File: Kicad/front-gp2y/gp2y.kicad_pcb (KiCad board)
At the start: 2 copper layers, 48 x 35 mm, 16 parts, among them IC1 MCP1755-50, K1 GP2Y, K2 MCU

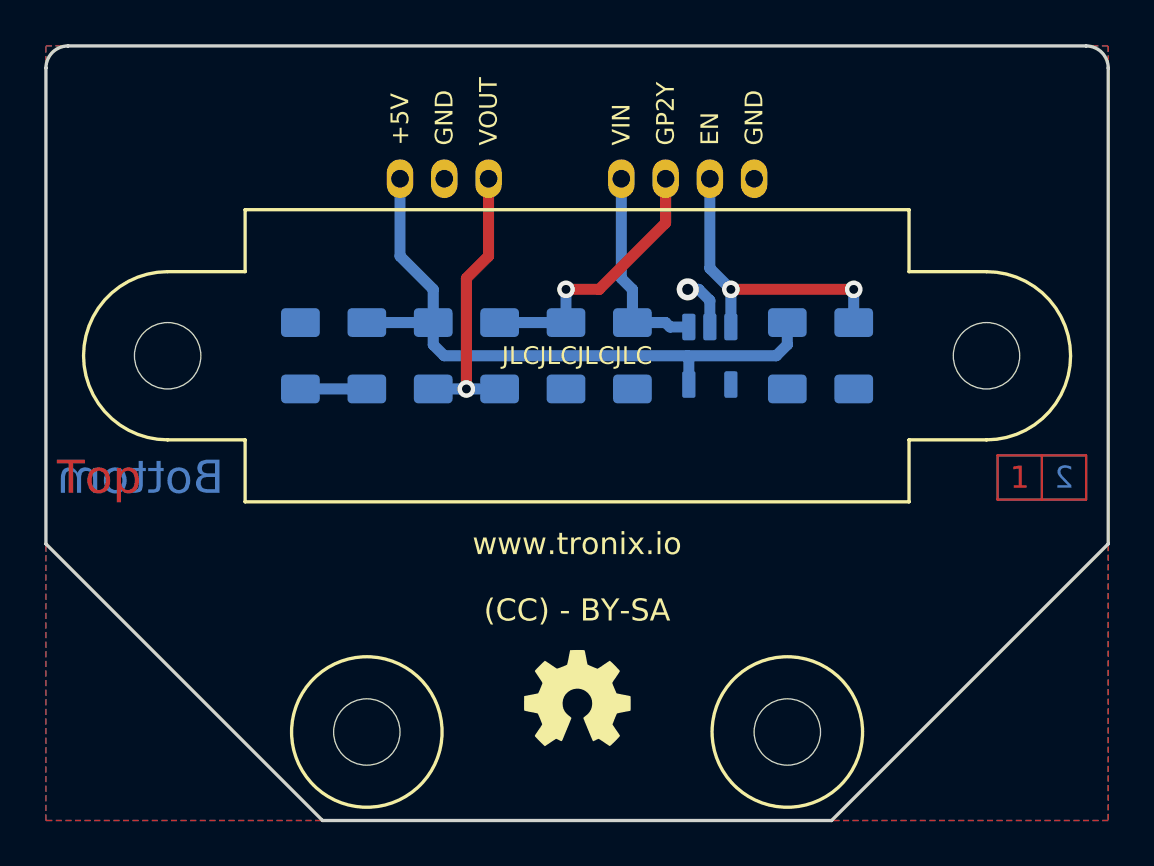
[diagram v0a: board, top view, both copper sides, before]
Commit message: Update GP2Y
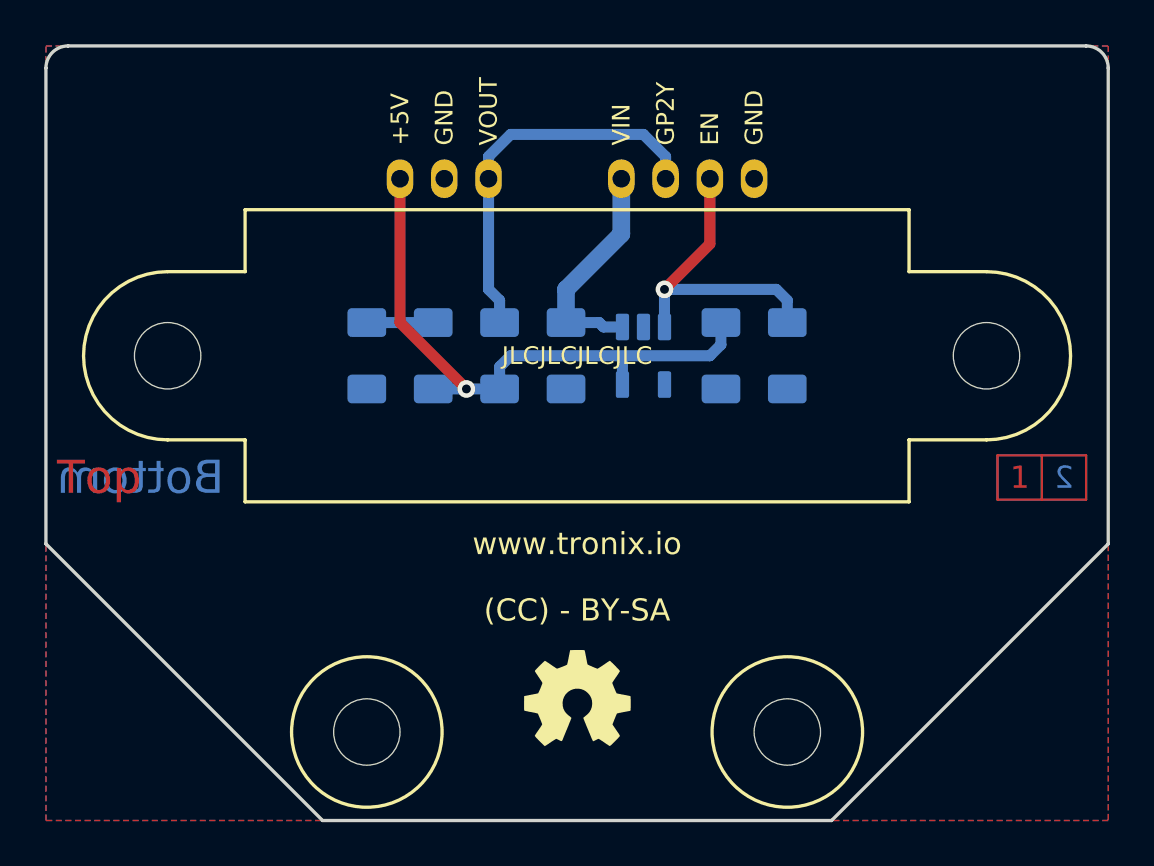
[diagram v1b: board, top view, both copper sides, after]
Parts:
- removed R4: NP, tronixio:RESISTOR-1206
- removed R5: 10K, tronixio:RESISTOR-1206
- R3: value 0Ω -> 10K
- moved C1 3.00 mm to (123.5, 79.0)
- moved C2 3.00 mm to (130.5, 79.0)
- moved IC1 3.00 mm to (127.0, 79.0)
- moved LED1 3.00 mm to (114.5, 79.0), turned to 90 degrees
- moved R1 3.00 mm to (133.5, 79.0)
- moved R2 3.00 mm to (117.5, 79.0), turned to 90 degrees
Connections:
- K2 pad 3: MCU_OUT -> GP2Y_OUT
- R3 pad 1: GP2Y_OUT -> +5V
- R3 pad 2: MCU_OUT -> GP2Y_OUT
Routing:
- net MCU_OUT: track 12.2 -> 0.00 mm, vias 1 -> 0
- net GP2Y_OUT: track 12.9 -> 17.5 mm, vias 1 -> 0
- net +5V: track 29.9 -> 27.4 mm, vias 0 -> 1
- net GND: track 2.41 -> 0.00 mm, vias 1 -> 0
- net VIN: track 9.34 -> 10.2 mm
- net MCU_ENABLE: track 14.1 -> 14.3 mm, vias 2 -> 1
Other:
- board text removed: "Output 3V3"
- board text removed: "Output 5V"

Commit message: Update gp2y.kicad_pcb
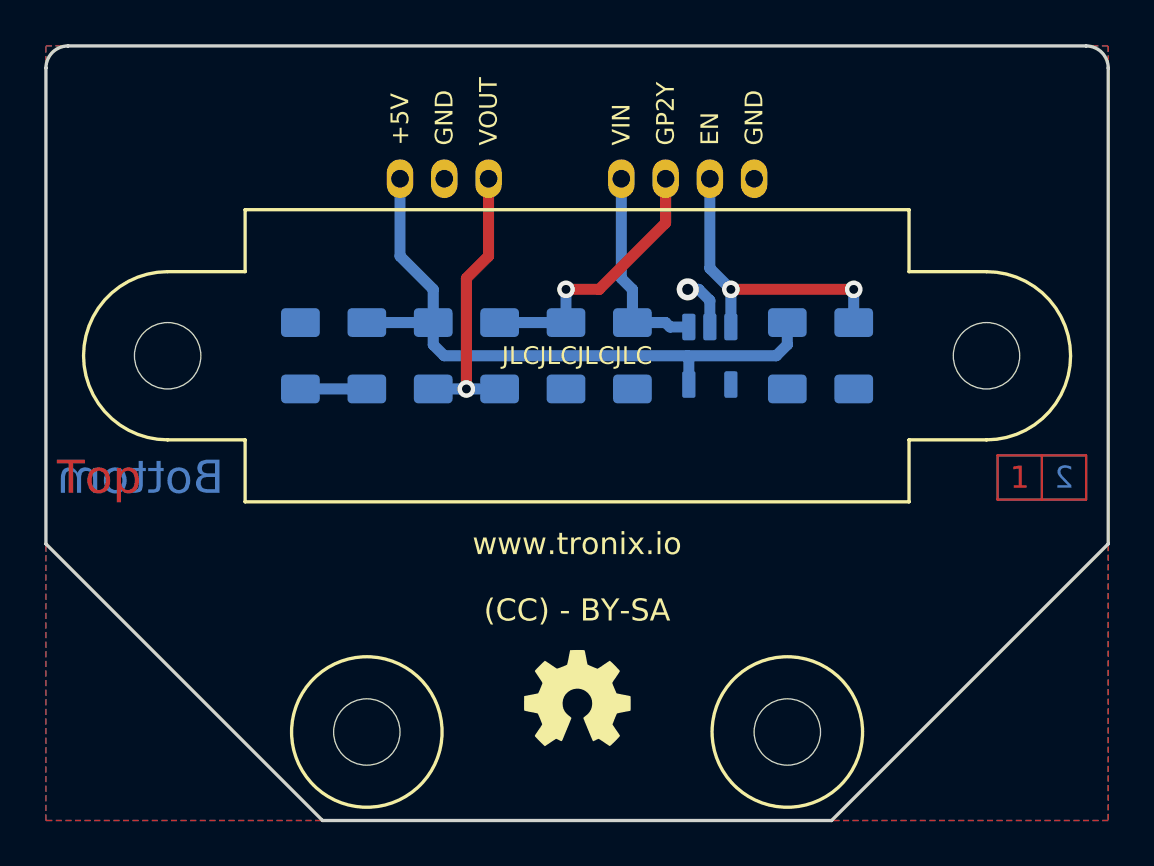
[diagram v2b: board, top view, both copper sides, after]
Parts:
- added R4: NP, tronixio:RESISTOR-1206, B.Cu at (123.5, 79.0)
- added R5: 10K, tronixio:RESISTOR-1206, B.Cu at (117.5, 79.0)
- R3: value 10K -> 0Ω
- moved C1 3.00 mm to (126.5, 79.0)
- moved C2 3.00 mm to (133.5, 79.0)
- moved IC1 3.00 mm to (130.0, 79.0)
- moved LED1 3.00 mm to (111.5, 79.0), turned to -90 degrees
- moved R1 3.00 mm to (136.5, 79.0)
- moved R2 3.00 mm to (114.5, 79.0), turned to -90 degrees
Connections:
- K2 pad 3: GP2Y_OUT -> MCU_OUT
- R3 pad 1: +5V -> GP2Y_OUT
- R3 pad 2: GP2Y_OUT -> MCU_OUT
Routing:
- net MCU_OUT: track 0.00 -> 12.2 mm, vias 0 -> 1
- net GP2Y_OUT: track 17.5 -> 12.9 mm, vias 0 -> 1
- net +5V: track 27.4 -> 29.9 mm, vias 1 -> 0
- net GND: track 0.00 -> 2.41 mm, vias 0 -> 1
- net VIN: track 10.2 -> 9.34 mm
- net MCU_ENABLE: track 14.3 -> 14.1 mm, vias 1 -> 2
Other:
- board text added: "Output 3V3"
- board text added: "Output 5V"
